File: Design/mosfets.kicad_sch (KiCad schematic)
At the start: 0 parts

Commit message: MOSFETS
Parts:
- added C? (x3): 2.2u, symbol Device:C_Small
- added Q? (x6): TPH2R608NH,L1Q, symbol Transistor_FET:AO3400A
- added R? (x6): 10, symbol Device:R_Small
- added R? (x6): 10k, symbol Device:R
- added R? (x3): 0.0005, symbol Device:R_Small
- added U? (x3): AD8418, symbol Amplifier_Current:AD8418
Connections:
- new net: Q?.1 (G), R?.2, R?.2 (x6)
- new net: Q?.2 (S), R?.1 (x6)
- new net: C?.2, U?.2 (GND), U?.3 (REF2) (x3)
- new net: R?.1, U?.1 (IN-) (x3)
- new net: R?.2, U?.8 (IN+) (x3)
- new net +3.3V: C?.1, C?.1, C?.1, U?.6 (VS), U?.6 (VS), U?.6 (VS), U?.7 (REF1), U?.7 (REF1), U?.7 (REF1)

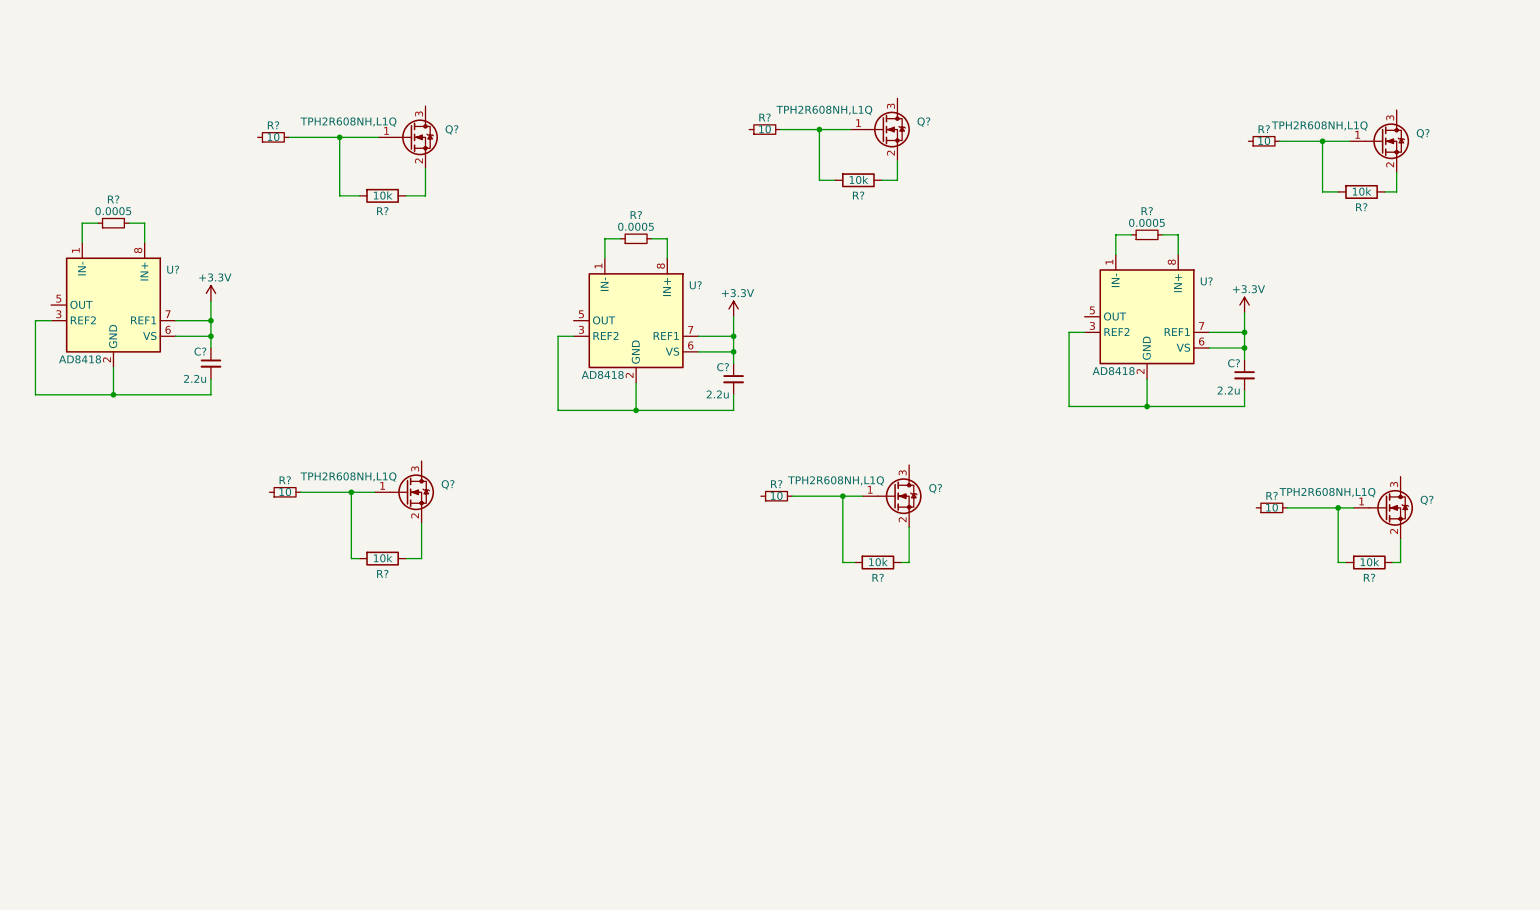
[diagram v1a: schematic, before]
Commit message: MOSFETs
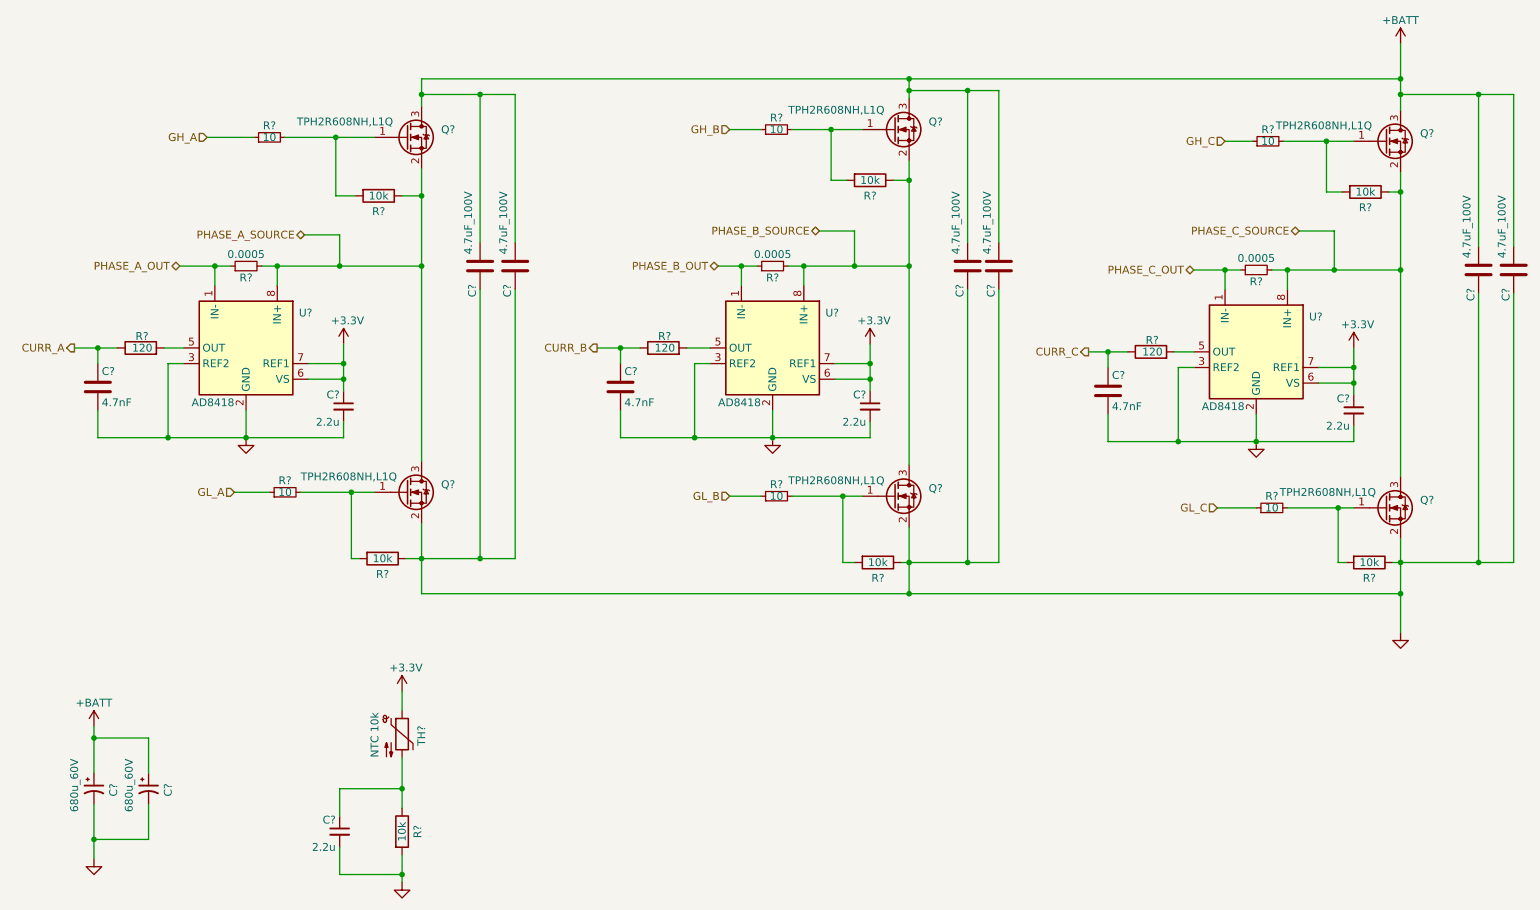
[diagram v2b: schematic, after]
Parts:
- added C? (x6): 4.7uF_100V, symbol Device:C
- added C? (x3): 4.7nF, symbol Device:C
- added C?: 2.2u, symbol Device:C_Small
- added C? (x2): 680u_60V, symbol Device:C_Polarized_Small_US
- added R?: 10k, symbol Device:R
- added R? (x3): 120, symbol Device:R
- added TH?: NTC 10k, symbol Device:Thermistor_NTC
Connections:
- net +3.3V: now also TH?.1
- net GH_C: now reaches R?.1
- net PHASE_B_SOURCE: now reaches Q?.2 (S), R?.1
- net PHASE_B_SOURCE: now also Q?.3 (D), R?.2, U?.8 (IN+)
- net +BATT: now reaches Q?.3 (D)
- net +BATT: now also Q?.3 (D), Q?.3 (D), C?.1, C?.1, C?.1, C?.1, C?.1, C?.1, C?.1, C?.1
- net GND: now reaches C?.2, U?.2 (GND), U?.3 (REF2)
- net GND: now also C?.2, C?.2, Q?.2 (S), Q?.2 (S), Q?.2 (S), R?.1, R?.1, R?.1, U?.2 (GND), U?.2 (GND), U?.3 (REF2), U?.3 (REF2), C?.2, C?.2, C?.2, C?.2, C?.2, C?.2, C?.2, C?.2, C?.2, C?.2, C?.2, C?.2, R?.2
- net PHASE_A_SOURCE: now reaches Q?.2 (S), R?.1
- net PHASE_A_SOURCE: now also Q?.3 (D), R?.2, U?.8 (IN+)
- net GH_A: now reaches R?.1
- net PHASE_B_OUT: now reaches R?.1, U?.1 (IN-)
- net at U?.5 (OUT): now also R?.2 (x3)
- net PHASE_C_SOURCE: now reaches Q?.3 (D)
- net PHASE_C_SOURCE: now also Q?.2 (S), R?.1, R?.2, U?.8 (IN+)
- net GL_A: now reaches R?.1
- net PHASE_C_OUT: now reaches R?.1, U?.1 (IN-)
- net GL_B: now reaches R?.1
- net GL_C: now reaches R?.1
- net GH_B: now reaches R?.1
- net PHASE_A_OUT: now reaches R?.1, U?.1 (IN-)
- new net: C?.1, R?.1, TH?.2
- new net CURR_A: C?.1, R?.1
- new net CURR_B: C?.1, R?.1
- new net CURR_C: C?.1, R?.1
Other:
- moved on the sheet: C?, Q?, R?, U?
